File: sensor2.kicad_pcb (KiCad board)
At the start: 2 copper layers, 95 x 72 mm, 36 parts, among them CON1 DC2.5-9V, CON2 AVR-ISP-6, CON3 DM3AT-SF-PEJM5, IC1 ATMEGA328P-P, J1 AE-STEREO-MINI, P1 D-SUB9, P2 GMS6-CR6, P3 BATT, Q1 2SC1815, SW1 STOP, SW2 TOGGLE, SW3 START, SW4 NEXT, U1 SL-TPS63060, U2 AE-LPS331AP, U3 SL-MPU9150, U4 SL-SB1602BW, X1 8MHz

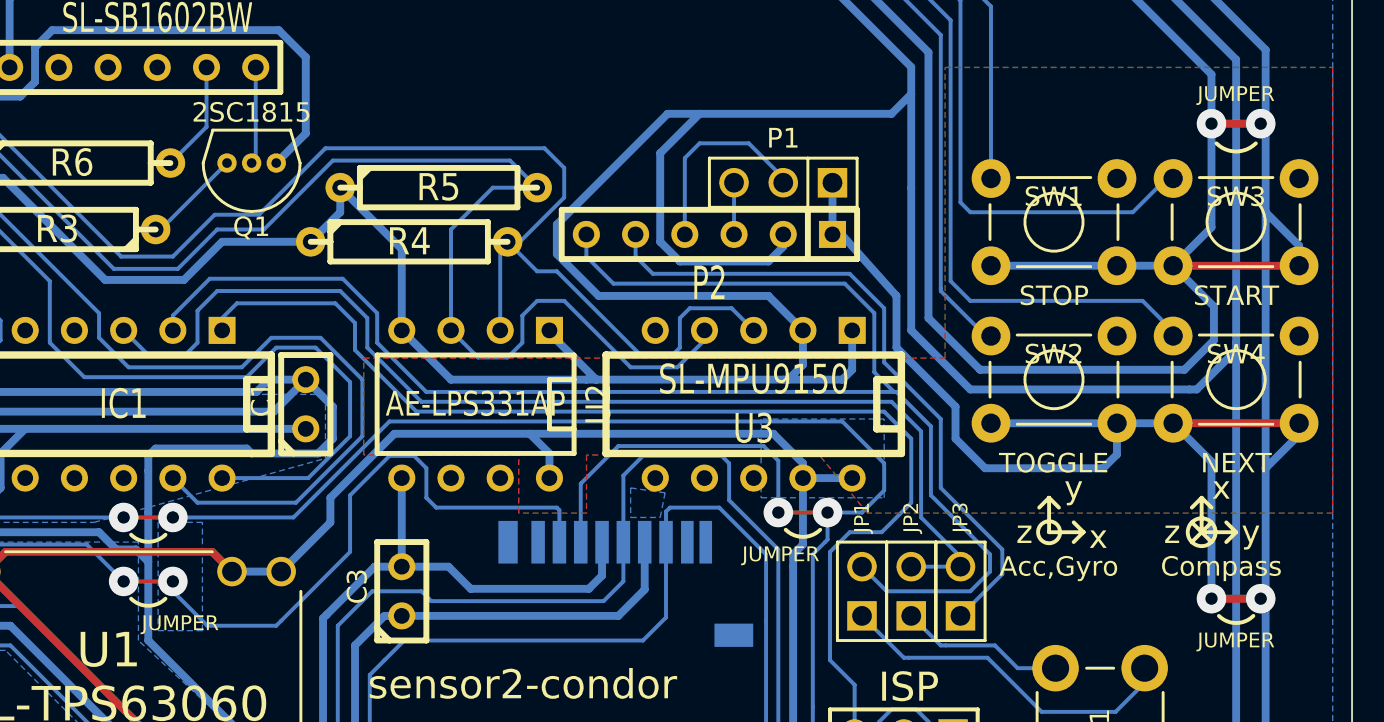
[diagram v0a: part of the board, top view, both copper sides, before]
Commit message: Release
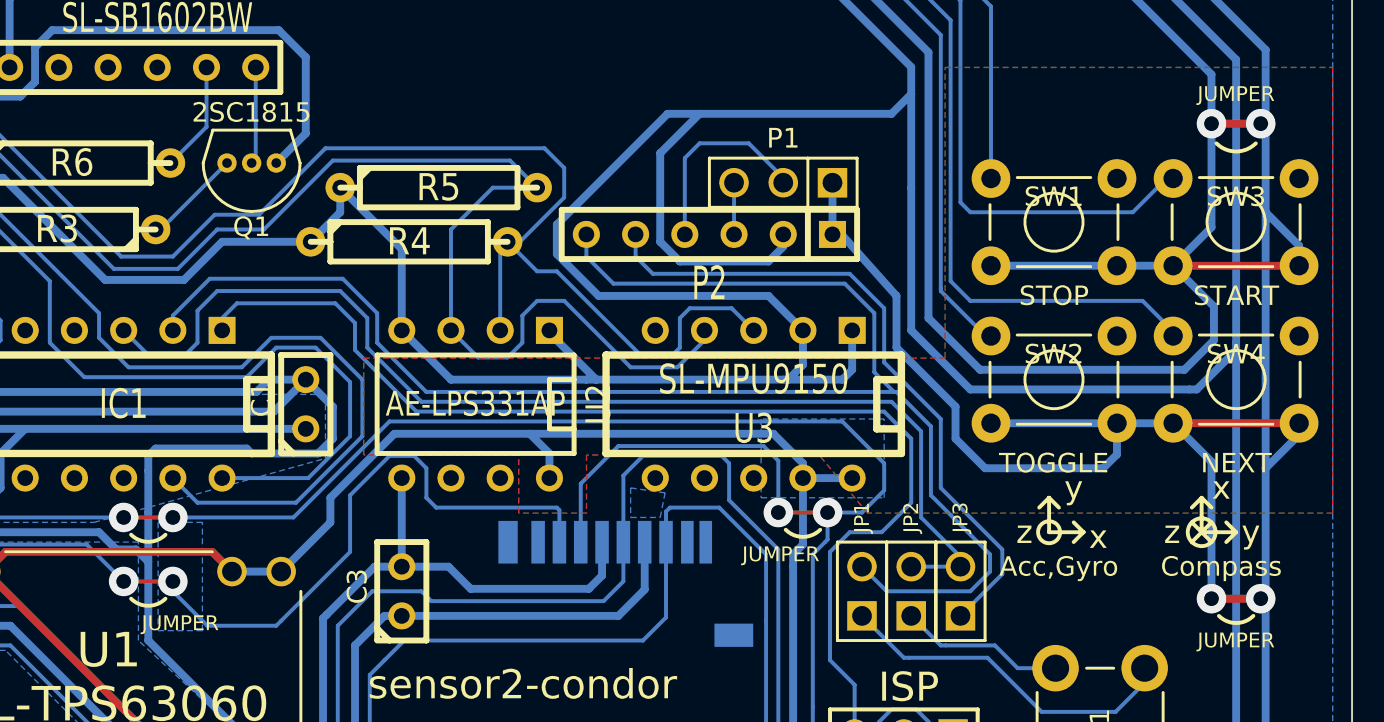
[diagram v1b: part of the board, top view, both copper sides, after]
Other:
- net class Bold: via_dia 0.889 -> 1.524; via_drill 0.635 -> 1.016
- net class Default: via_dia 0.889 -> 1.524; via_drill 0.635 -> 1.016
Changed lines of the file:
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@@
     (segment_width 0.2)
     (edge_width 0.1)
-    (via_size 0.889)
-    (via_drill 0.635)
+    (via_size 1.524)
+    (via_drill 1.016)
     (via_min_size 0.889)
     (via_min_drill 0.6096)
@@
       (drillshape 0)
       (scaleselection 1)
-      (outputdirectory garber/))
+      (outputdirectory gerber/))
   )
   (net 0 "")
@@
     (clearance 0.2032)
     (trace_width 0.2032)
-    (via_dia 0.889)
-    (via_drill 0.635)
+    (via_dia 1.524)
+    (via_drill 1.016)
     (uvia_dia 0.508)
     (uvia_drill 0.127)
@@
     (clearance 0.2032)
     (trace_width 0.4064)
-    (via_dia 0.889)
-    (via_drill 0.635)
+    (via_dia 1.524)
+    (via_drill 1.016)
     (uvia_dia 0.508)
     (uvia_drill 0.127)
